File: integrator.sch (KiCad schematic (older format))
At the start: 22 parts, among them J1 SJ-3524-SMT, J2 SJ-3524-SMT, SW1 EVQP40B3M, SW2 EVQP40B3M, U1 Teensy3.2, U2 ICM-20600

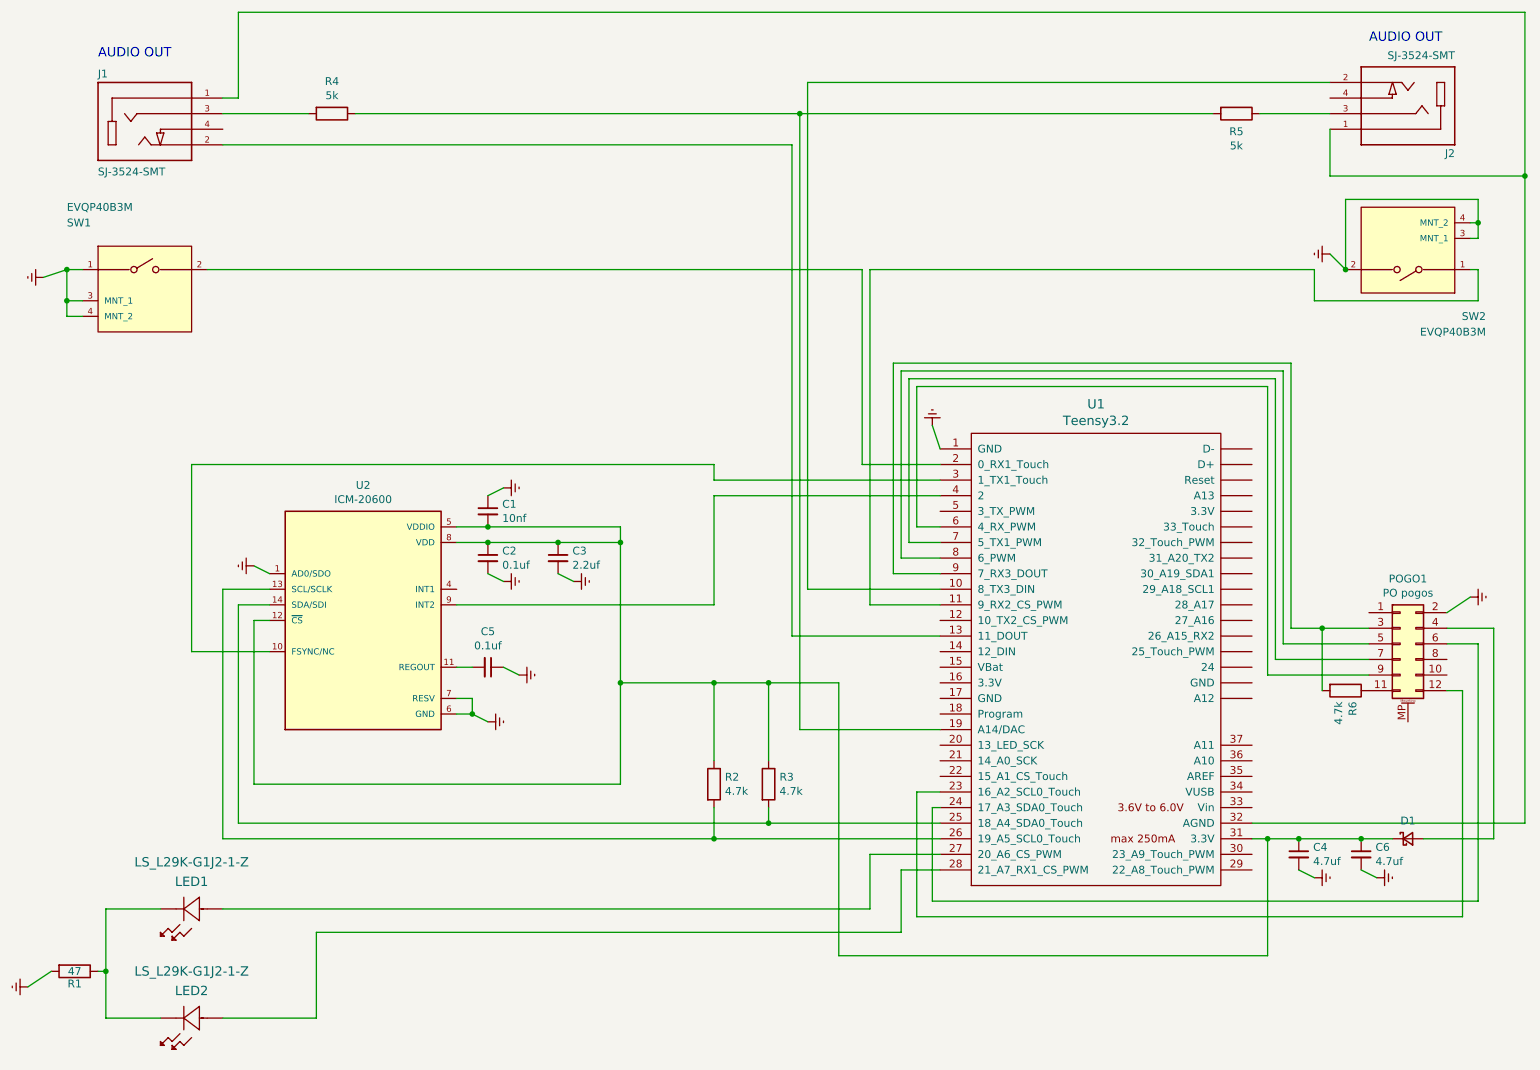
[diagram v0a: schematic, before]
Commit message: last changes of rev3
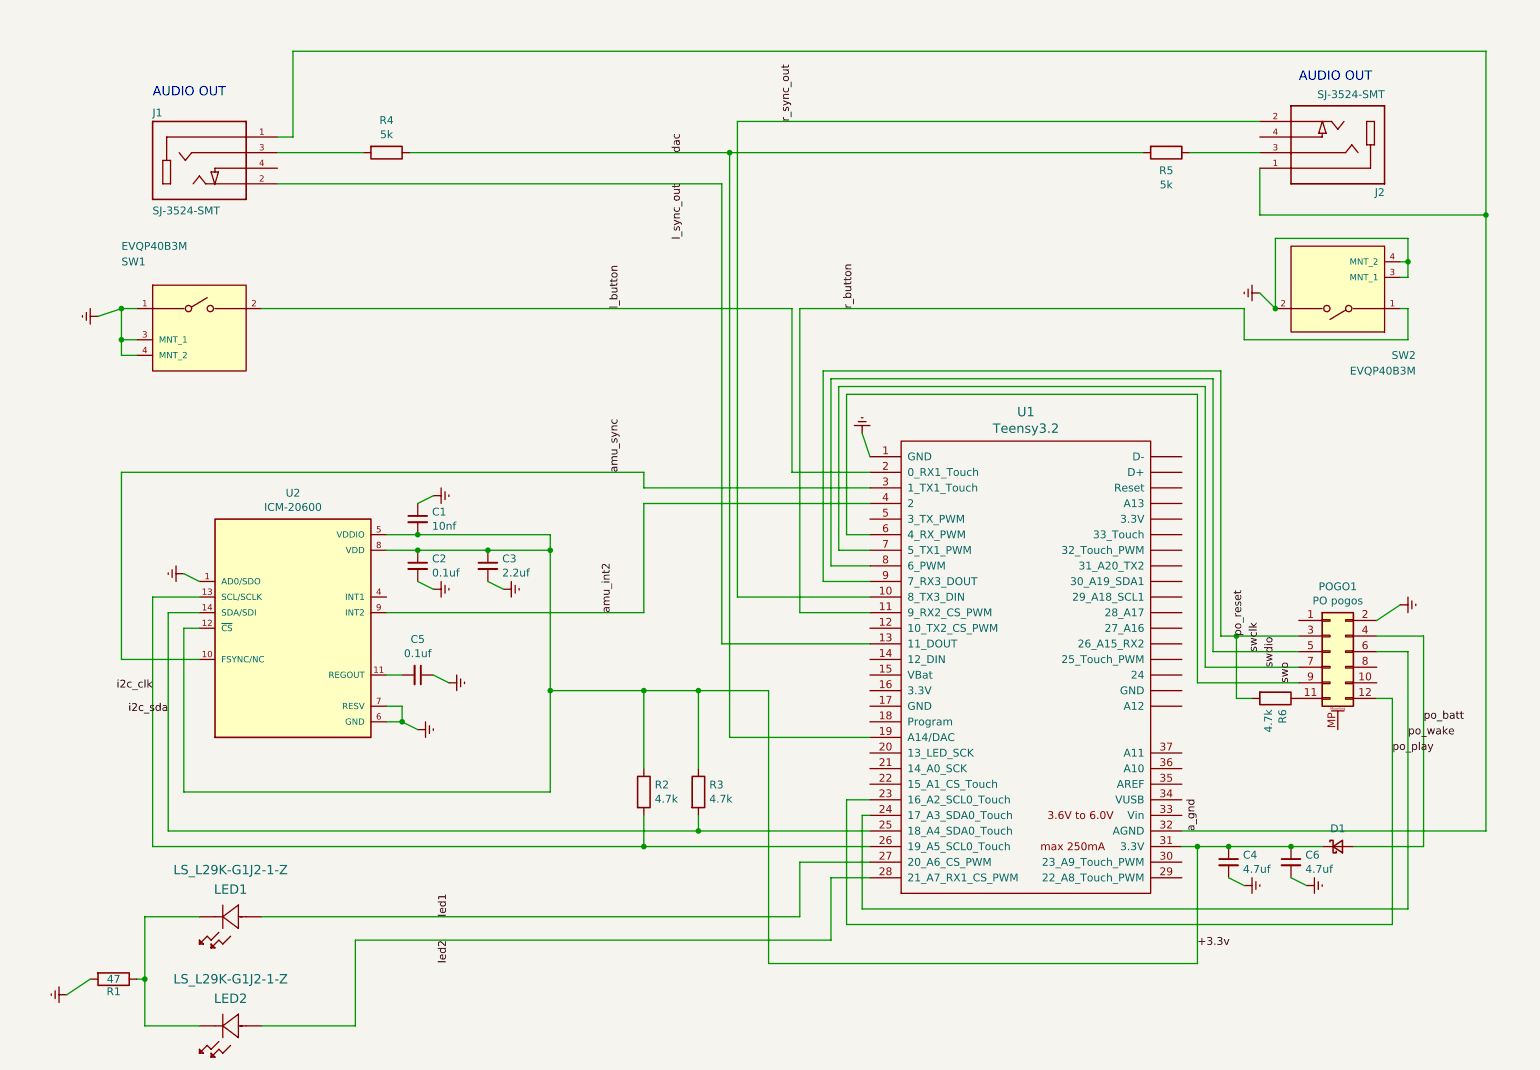
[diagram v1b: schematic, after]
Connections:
- net r_sync_out: now reaches J2.2, U1.10 (8_TX3_DIN)
- net r_button: now reaches SW2.1, U1.11 (9_RX2_CS_PWM)
- net l_sync_out: now reaches J1.2, U1.13 (11_DOUT)
- net dac: now reaches R4.1, R5.2, U1.19 (A14/DAC)
- net l_button: now reaches SW1.2, U1.2 (0_RX1_Touch)
- net po_play: now reaches POGO1.12 (Pin_12), U1.23 (16_A2_SCL0_Touch)
- net po_wake: now reaches POGO1.6 (Pin_6), U1.24 (17_A3_SDA0_Touch)
- net i2c_sda: now reaches R3.2, U1.25 (18_A4_SDA0_Touch), U2.14 (SDA/SDI)
- net i2c_clk: now reaches R2.2, U1.26 (19_A5_SCL0_Touch), U2.13 (SCL/SCLK)
- net led1: now reaches LED1.2, U1.27 (20_A6_CS_PWM)
- net led2: now reaches LED2.2, U1.28 (21_A7_RX1_CS_PWM)
- net amu_sync: now reaches U1.3 (1_TX1_Touch), U2.10 (FSYNC/NC)
- net +3.3v: now reaches C1.2, C2.1, C3.1, C4.1, C6.1, D1.1 (K), R2.1, R3.1, U1.31 (3.3V), U2.12 (~CS), U2.5 (VDDIO), U2.8 (VDD)
- net a_gnd: now reaches J1.1, J2.1, U1.32 (AGND)
- net amu_int2: now reaches U1.4 (2), U2.9 (INT2)
- net swo: now reaches POGO1.9 (Pin_9), U1.6 (4_RX_PWM)
- net swdio: now reaches POGO1.7 (Pin_7), U1.7 (5_TX1_PWM)
- net swclk: now reaches POGO1.5 (Pin_5), U1.8 (6_PWM)
- net po_reset: now reaches POGO1.3 (Pin_3), R6.2, U1.9 (7_RX3_DOUT)
- net po_batt: now reaches D1.2 (A), POGO1.4 (Pin_4)
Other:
- moved on the sheet: C1, C2, C3, C4, C5, C6, D1, J1, J2, LED1, LED2, POGO1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
